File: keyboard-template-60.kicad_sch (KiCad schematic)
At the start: 175 parts, among them J1 USB_C_Receptacle_USB2.0, J2 Conn_01x04_MountingPin, J3 AVR-ISP-6, SW1 SW_Reset, U1 ATmega32U4-M, U2 SRV05-4, Y1 16MHz

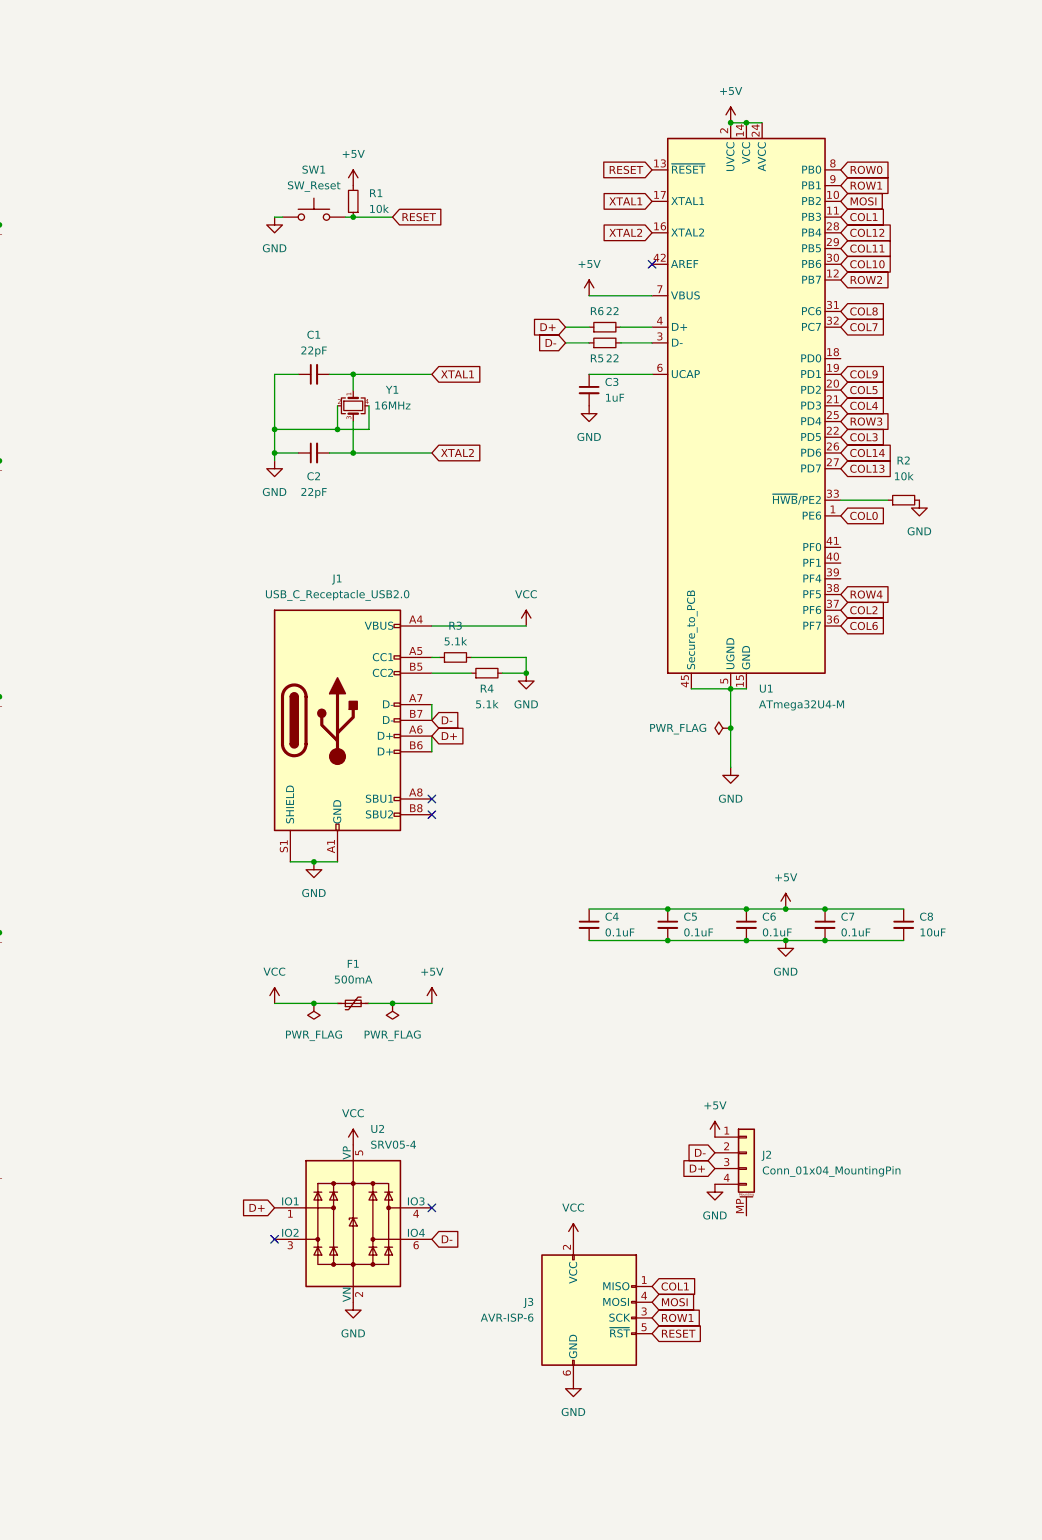
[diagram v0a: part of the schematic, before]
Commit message: introduce trackpoint files and placement - VERY ROUGH WIP
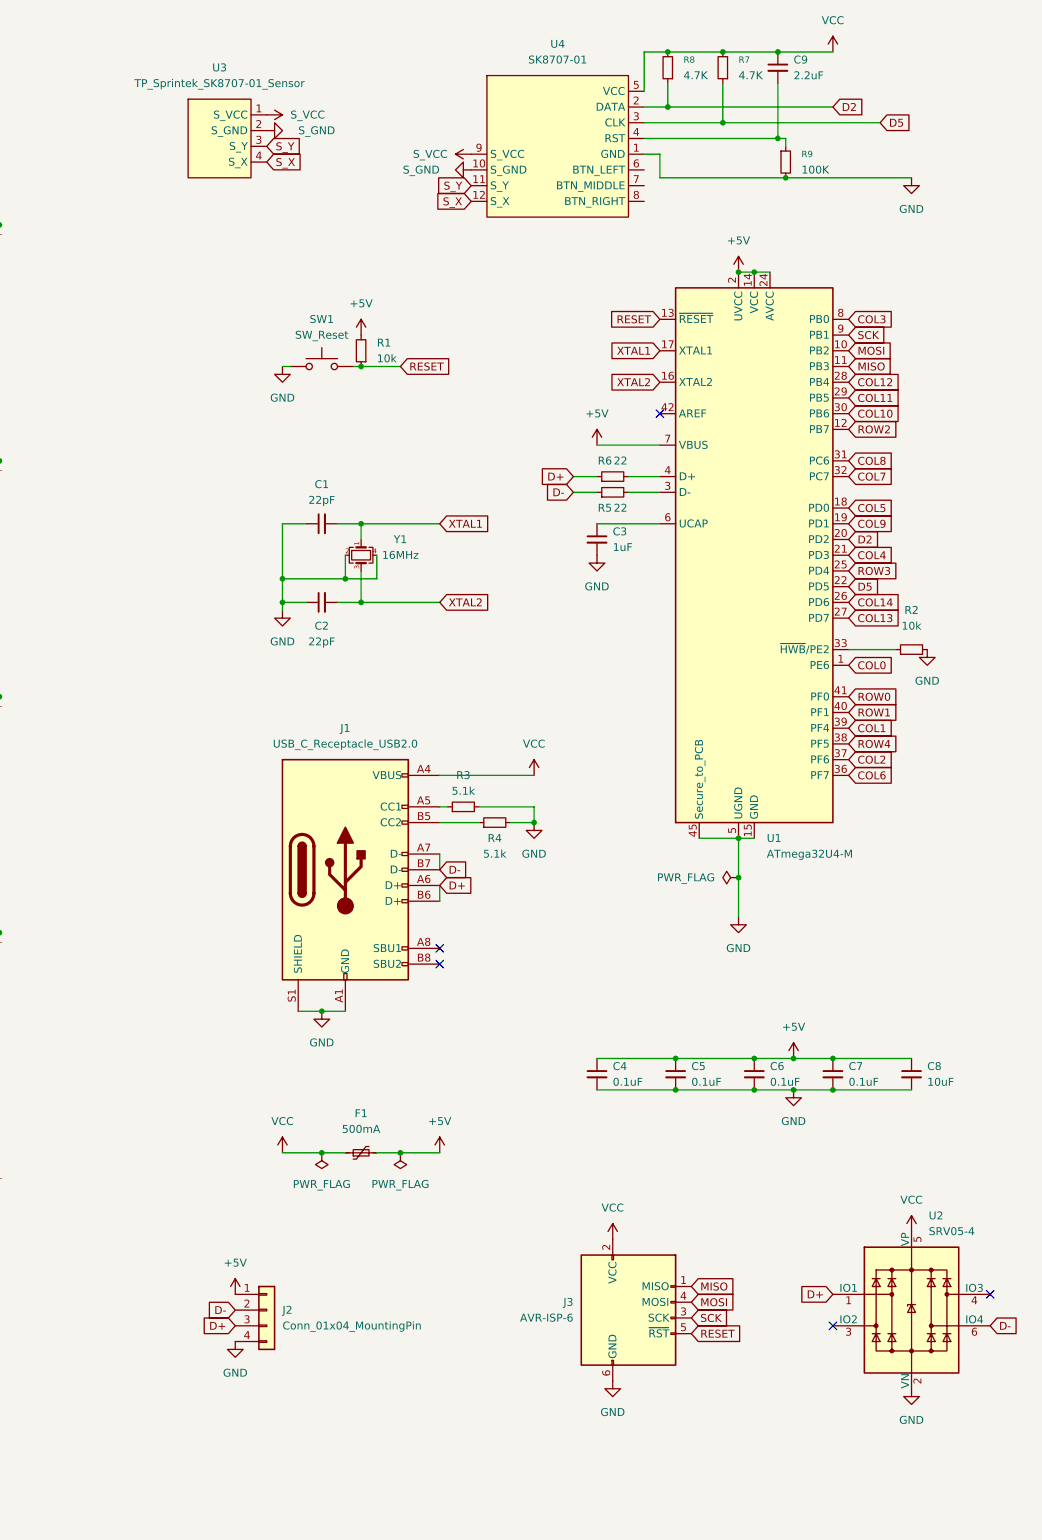
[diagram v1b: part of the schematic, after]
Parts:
- added C9: 2.2uF, Capacitor_SMD:C_0603_1608Metric_Pad1.08x0.95mm_HandSolder, symbol Device:C_Small
- added R7, R8: 4.7K, Capacitor_SMD:C_0603_1608Metric_Pad1.08x0.95mm_HandSolder, symbol Device:R_Small
- added R9: 100K, Capacitor_SMD:C_0603_1608Metric_Pad1.08x0.95mm_HandSolder, symbol Device:R_Small
- added U3: TP_Sprintek_SK8707-01_Sensor, ssbb_parts:TP_Sprintek_SK8707-01_Sensor_reversible, symbol ssbb_parts:TP_Sprintek_SK8707-01_Sensor
- added U4: SK8707-01, ssbb_parts:TP_Sprintek_SK8707-01_reversible, symbol ssbb_parts:TP_Sprintek_SK8707–01
- H1, H2, H3, H4, H5, H6: footprint MountingHole:MountingHole_2.2mm_M2_Pad_TopOnly -> MountingHole:MountingHole_2.5mm
- J2: symbol Connector_Generic_MountingPin:Conn_01x04_MountingPin -> Connector_Generic:Conn_01x04
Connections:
- net COL1: now also U1.39 (PF4); no longer J3.1 (MISO), U1.11 (PB3)
- net COL3: now also U1.8 (PB0); no longer U1.22 (PD5)
- net COL5: now also U1.18 (PD0); no longer U1.20 (PD2)
- net GND: now also R9.2, U4.1 (GND)
- net ROW0: now also U1.41 (PF0); no longer U1.8 (PB0)
- net ROW1: now also U1.40 (PF1); no longer J3.3 (SCK), U1.9 (PB1)
- net VCC: now also C9.1, R7.2, R8.2, U4.5 (VCC)
- new net: C9.2, R9.1, U4.4 (RST)
- new net D2: R8.1, U1.20 (PD2), U4.2 (DATA)
- new net D5: R7.1, U1.22 (PD5), U4.3 (CLK)
- new net MISO: J3.1 (MISO), U1.11 (PB3)
- new net SCK: J3.3 (SCK), U1.9 (PB1)
- new net S_GND: U3.2 (S_GND), U4.10 (S_GND)
- new net S_VCC: U3.1 (S_VCC), U4.9 (S_VCC)
- new net S_X: U3.4 (S_X), U4.12 (S_X)
- new net S_Y: U3.3 (S_Y), U4.11 (S_Y)
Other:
- moved on the sheet: C1, C2, C3, C4, C5, C6, C7, C8, F1, J1, J3, R1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
